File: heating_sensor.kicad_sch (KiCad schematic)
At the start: 3 parts

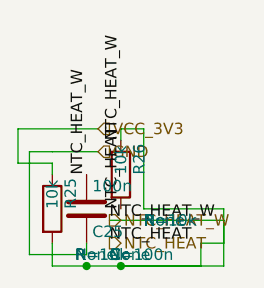
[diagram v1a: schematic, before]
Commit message: fix
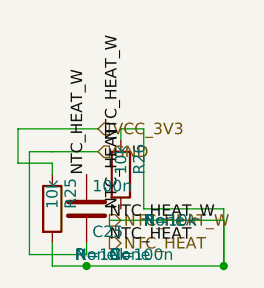
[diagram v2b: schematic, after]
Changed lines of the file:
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@@
 				(instances
 			(project "climate_control_niva_travel"
-				(path "/a20a8d43-2e18-4318-8ef3-7f434a470dab/1469a1ed-0edc-4b26-9fa4-af555b72a5f7"(reference "C0425") (unit 1) )
+				(path "/d978731e-2b44-43df-ac1e-7ebc58fad63b"(reference "C25") (unit 1) )
+				(path "/aece091b-8e26-4b21-9786-1b0efc647a51/25ffff2c-bc01-4b6e-82ac-0a5cb114cf15"(reference "C0425") (unit 1) )
 			)
 		)
@@
 				(instances
 			(project "climate_control_niva_travel"
-				(path "/a20a8d43-2e18-4318-8ef3-7f434a470dab/1469a1ed-0edc-4b26-9fa4-af555b72a5f7"(reference "R0425") (unit 1) )
+				(path "/d978731e-2b44-43df-ac1e-7ebc58fad63b"(reference "R25") (unit 1) )
+				(path "/aece091b-8e26-4b21-9786-1b0efc647a51/25ffff2c-bc01-4b6e-82ac-0a5cb114cf15"(reference "R0425") (unit 1) )
 			)
 		)
@@
 				(instances
 			(project "climate_control_niva_travel"
-				(path "/a20a8d43-2e18-4318-8ef3-7f434a470dab/1469a1ed-0edc-4b26-9fa4-af555b72a5f7"(reference "R0426") (unit 1) )
+				(path "/d978731e-2b44-43df-ac1e-7ebc58fad63b"(reference "R26") (unit 1) )
+				(path "/aece091b-8e26-4b21-9786-1b0efc647a51/25ffff2c-bc01-4b6e-82ac-0a5cb114cf15"(reference "R0426") (unit 1) )
 			)
 		)
@@
 	(wire
 		(pts
-			(xy 33.02 17.78) (xy 33.02 21.59)
-		)
-		(stroke
-			(width 0)
-			(type default)
-		)
-	)
-	(wire
-		(pts
-			(xy 33.02 21.59) (xy 30.48 21.59)
-		)
-		(stroke
-			(width 0)
-			(type default)
-		)
-	)
-	(wire
-		(pts
-			(xy 30.48 21.59) (xy 30.48 24.13)
-		)
-		(stroke
-			(width 0)
-			(type default)
-		)
-	)
-	(wire
-		(pts
-			(xy 30.48 24.13) (xy 21.59 24.13)
+			(xy 33.02 17.78) (xy 33.02 24.13)
 		)
 		(stroke
@@
 	)
 	(junction
-		(at 21.59 24.13)
+		(at 33.02 24.13)
 		(diameter 0.0000)
 		(color 0 0 0 0)
